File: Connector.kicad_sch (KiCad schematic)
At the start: 1 part, among them J6 2-338069-0

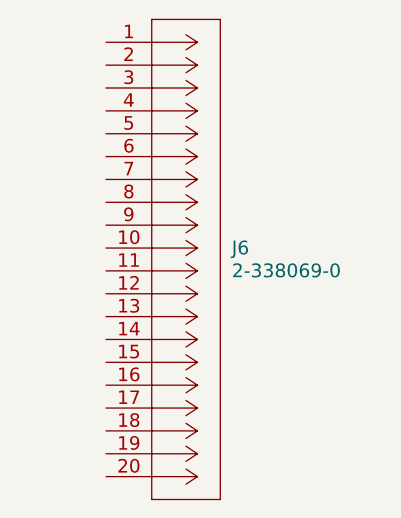
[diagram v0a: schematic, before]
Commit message: Стартовый вариант
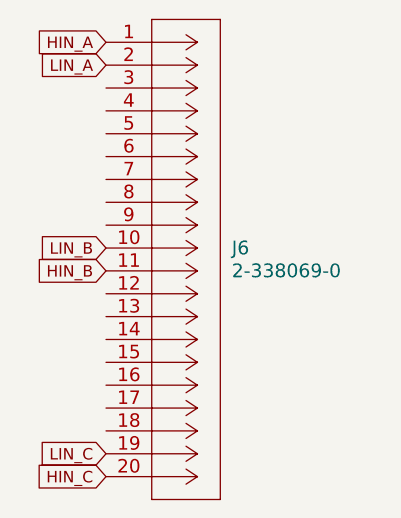
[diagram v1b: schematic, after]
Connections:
- net HIN_A: now reaches J6.1
- net LIN_B: now reaches J6.10
- net HIN_B: now reaches J6.11
- net LIN_C: now reaches J6.19
- net LIN_A: now reaches J6.2
- net HIN_C: now reaches J6.20
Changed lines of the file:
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@@
 (kicad_sch (version 20230121) (generator eeschema)
   (paper "A4")
+  (global_label "HIN_C" (shape input) (at 132.08 111.76 180) (fields_autoplaced)
+    (effects (font (size 1.27 1.27)) (justify right))
+    (property "Intersheetrefs" "${INTERSHEET_REFS}" (at 123.5914 111.76 0)
+      (effects (font (size 1.27 1.27)) (justify right) hide)
+    )
+  )
+  (global_label "LIN_B" (shape input) (at 132.08 86.36 180) (fields_autoplaced)
+    (effects (font (size 1.27 1.27)) (justify right))
+    (property "Intersheetrefs" "${INTERSHEET_REFS}" (at 123.8938 86.36 0)
+      (effects (font (size 1.27 1.27)) (justify right) hide)
+    )
+  )
+  (global_label "LIN_C" (shape input) (at 132.08 109.22 180) (fields_autoplaced)
+    (effects (font (size 1.27 1.27)) (justify right))
+    (property "Intersheetrefs" "${INTERSHEET_REFS}" (at 123.8938 109.22 0)
+      (effects (font (size 1.27 1.27)) (justify right) hide)
+    )
+  )
+  (global_label "HIN_A" (shape input) (at 132.08 63.5 180) (fields_autoplaced)
+    (effects (font (size 1.27 1.27)) (justify right))
+    (property "Intersheetrefs" "${INTERSHEET_REFS}" (at 123.7728 63.5 0)
+      (effects (font (size 1.27 1.27)) (justify right) hide)
+    )
+  )
+  (global_label "HIN_B" (shape input) (at 132.08 88.9 180) (fields_autoplaced)
+    (effects (font (size 1.27 1.27)) (justify right))
+    (property "Intersheetrefs" "${INTERSHEET_REFS}" (at 123.5914 88.9 0)
+      (effects (font (size 1.27 1.27)) (justify right) hide)
+    )
+  )
+  (global_label "LIN_A" (shape input) (at 132.08 66.04 180) (fields_autoplaced)
+    (effects (font (size 1.27 1.27)) (justify right))
+    (property "Intersheetrefs" "${INTERSHEET_REFS}" (at 124.0752 66.04 0)
+      (effects (font (size 1.27 1.27)) (justify right) hide)
+    )
+  )
   (symbol (lib_id "Connector_My:2-338069-0") (at 132.08 63.5 0) (unit 1)
     (in_bom yes) (on_board yes) (dnp no) (fields_autoplaced)
